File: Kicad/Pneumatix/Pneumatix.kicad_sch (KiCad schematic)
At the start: 16 parts, among them J1 436500404, J2 142-0701-801, J3 Conn_01x04_Socket, U1 E22-400T33S

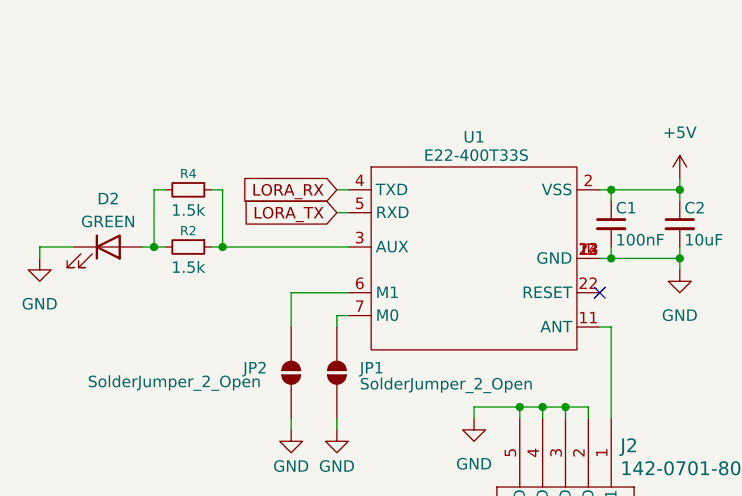
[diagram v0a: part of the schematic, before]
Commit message: wip: pcb components
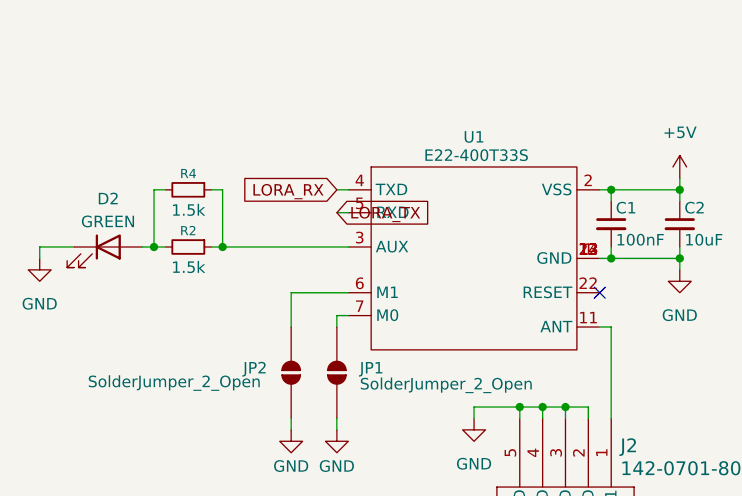
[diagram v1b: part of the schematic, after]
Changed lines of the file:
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@@
 	(global_label "LORA_TX"
 		(shape input)
-		(at 128.27 81.28 180)
+		(at 128.27 81.28 0)
 		(fields_autoplaced yes)
 		(effects
@@
 				(size 1.27 1.27)
 			)
-			(justify right)
+			(justify left)
 		)
 		(property "Intersheetrefs" "${INTERSHEET_REFS}"
-			(at 117.4229 81.28 0)
+			(at 139.1171 81.28 0)
 			(hide yes)
 			(show_name no)
@@
 					(size 1.27 1.27)
 				)
-				(justify right)
+				(justify left)
 			)
 		)
